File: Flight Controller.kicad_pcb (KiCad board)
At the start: 4 copper layers, 39.5 x 39.5 mm, 95 parts, among them IC2 AT7456E, J1 Conn_01x08_MountingPin, J2 USB_C_Receptacle_USB2.0_14P, Q2 BC817W, U1 AT32F435RGT7, U2 LMR51430, U3 BMP280, U4 SPX3819M5-L-3-3, U5 LMR51430, U6 W25Q128JVSIQ TR, U7 ICM-42688-P, U8 SPX3819M5-L-3-3, Y1 8M, Y2 27M

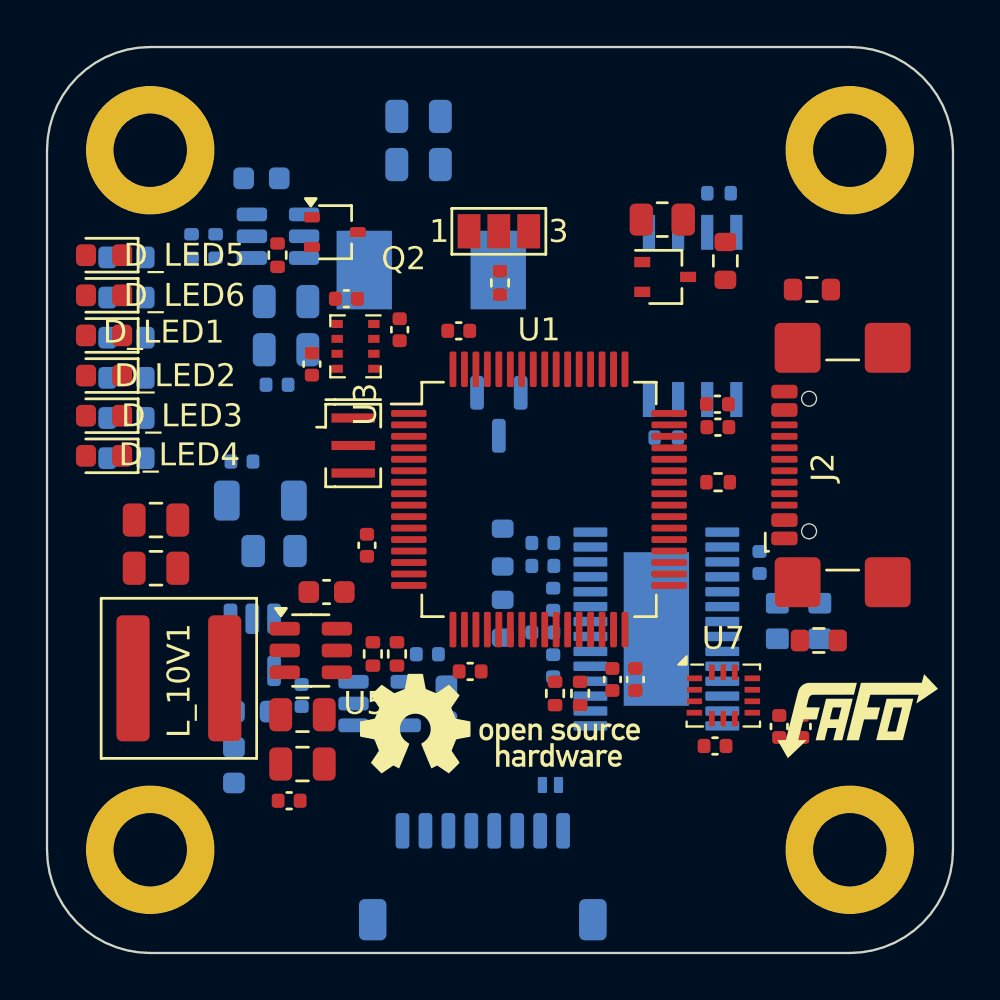
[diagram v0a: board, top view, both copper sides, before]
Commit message: Routing
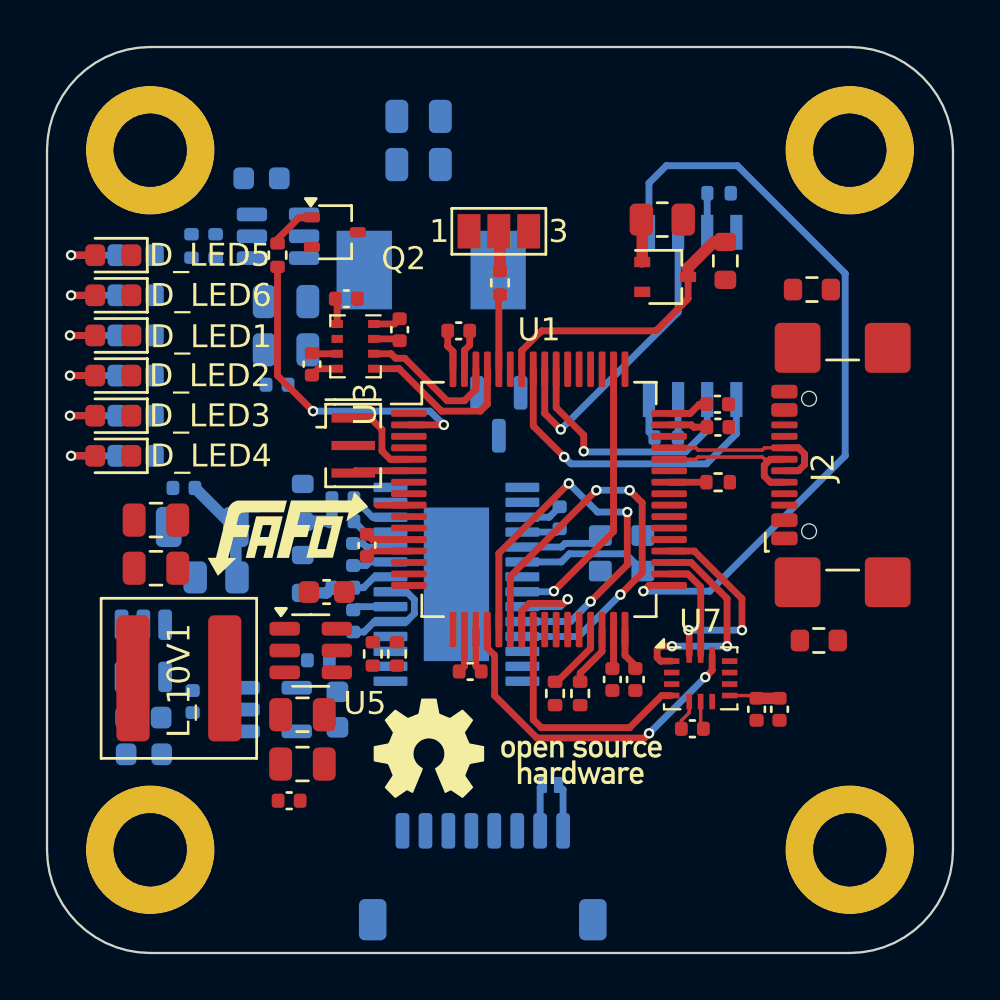
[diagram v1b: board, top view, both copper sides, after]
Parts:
- moved G*** 26.1 mm to (135.8, 86.5)
- moved C_OSD1 8.93 mm to (147.6, 85.8)
- moved C_OSD2 8.93 mm to (138.2, 85.0)
- moved C_OSD3 8.93 mm to (138.2, 86.0)
- moved C_OSD4 8.93 mm to (138.6, 87.5)
- moved C_OSD6 8.93 mm to (138.6, 90.3)
- moved IC2 8.93 mm to (143.1, 88.8)
- moved R_OSD1 8.93 mm to (136.4, 85.2)
- moved R_OSD2 8.93 mm to (136.4, 88.3)
- moved C_OSD5 8.93 mm to (138.2, 88.9)
- moved Y2 8.26 mm to (150.3, 87.4)
- moved C_3V1 4.76 mm to (129.4, 94.6)
- moved C_3V2 4.76 mm to (131.6, 93.9)
- moved C_3VG1 4.76 mm to (137.9, 94.2)
- moved C_3VG2 4.76 mm to (137.1, 92.1)
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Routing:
- net /FLASH_CS: track 0.00 -> 33.4 mm, vias 0 -> 1
- net /OSD_MISO: track 0.00 -> 19.3 mm, vias 0 -> 3
- net /OSD_SCLK: track 0.00 -> 18.6 mm, vias 0 -> 3
- net +3.3V: track 0.00 -> 16.7 mm
- net GND: track 0.00 -> 16.4 mm
- net /GYRO_CS: track 0.00 -> 15.1 mm, vias 0 -> 2
- net /BUZ: track 0.00 -> 14.4 mm, vias 0 -> 2
- net /FLASH_MOSI: track 0.00 -> 14.1 mm, vias 0 -> 1
- net /FLASH_MISO: track 0.00 -> 13.6 mm, vias 0 -> 1
- net /UART1_TX: track 0.00 -> 12.4 mm
- net /OSD_CS: track 0.00 -> 12.1 mm, vias 0 -> 1
- net /FLASH_SCLK: track 0.00 -> 11.2 mm, vias 0 -> 1
- net /GYRO_INT: track 0.00 -> 10.7 mm
- net /GYRO_MISO: track 0.00 -> 9.42 mm, vias 0 -> 2
- net /GYRO_MOSI: track 0.00 -> 8.84 mm, vias 0 -> 2
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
